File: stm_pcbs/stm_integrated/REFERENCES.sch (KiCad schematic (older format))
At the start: 20 parts, among them U13 AD8676, U14 AD8675, U15 ADR445

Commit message: working on Kicad of 3rd Dec
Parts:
- C65, C66, C69, C70, C71, C74: symbol CP2 -> device:CP1
- C67, C68, C72, C73, C75, C76: symbol C -> device:C
- R5, R6, R7, R8, R9: symbol R -> device:R
- U13: symbol AD8676 -> ad5791:AD8676
- U14: symbol AD8675 -> ad5791:AD8675
- U15: symbol adr445 -> adr445:adr445
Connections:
- wire segments 65 -> 81

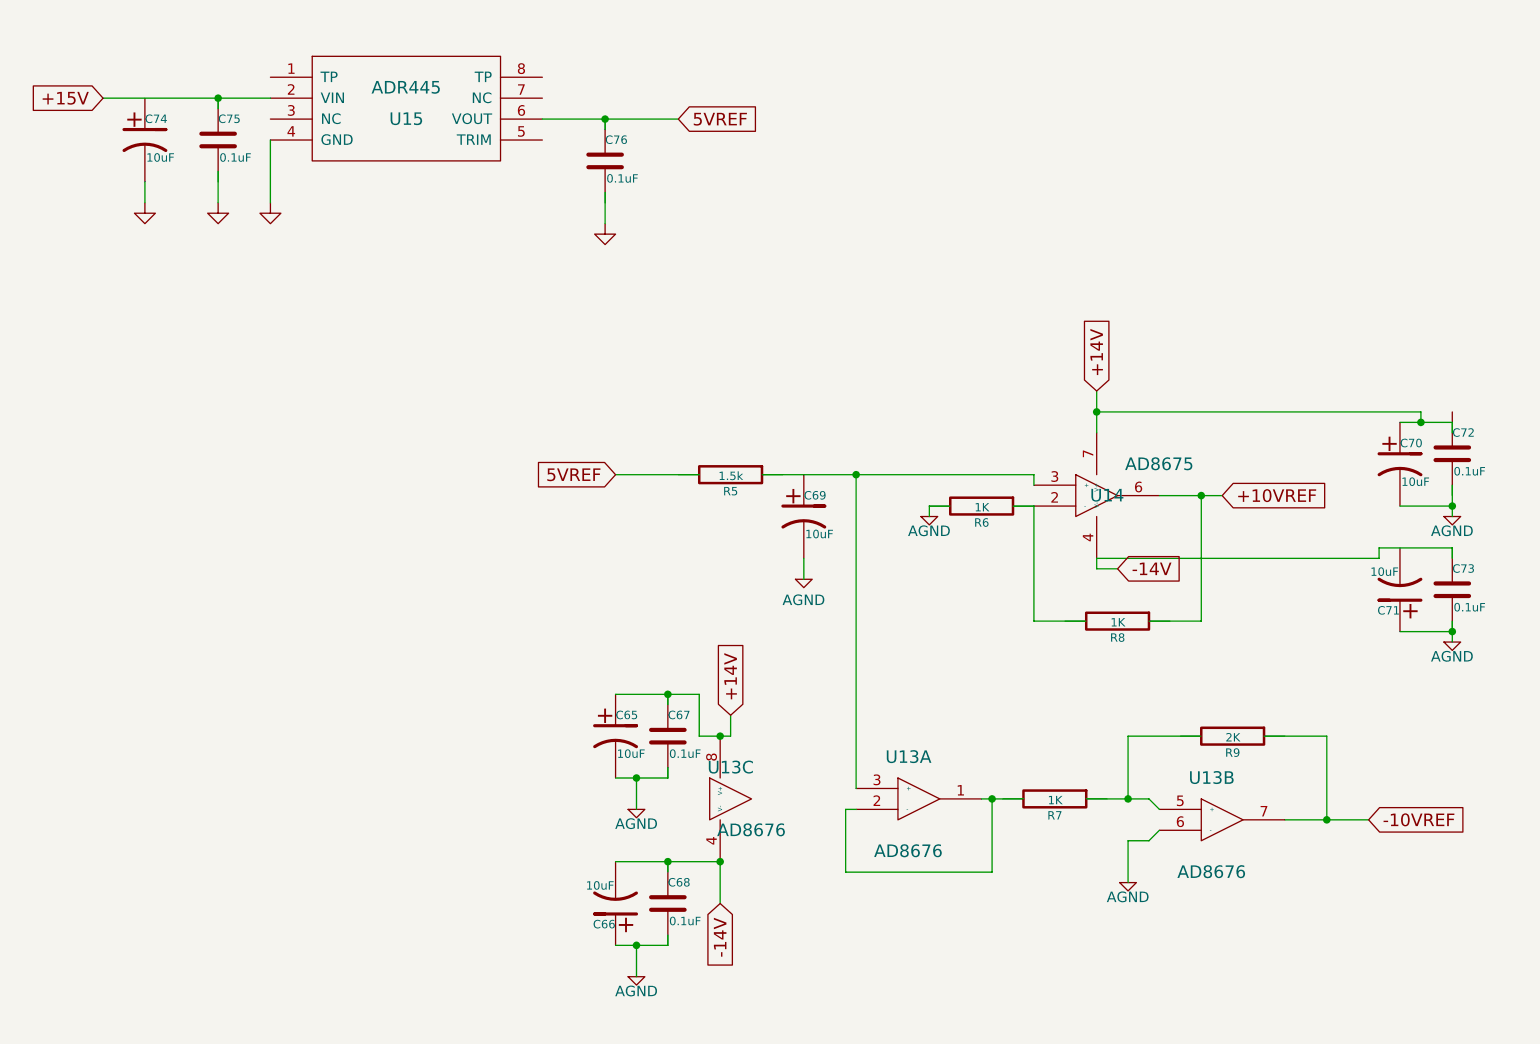
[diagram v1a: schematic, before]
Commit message: fixing more borkage
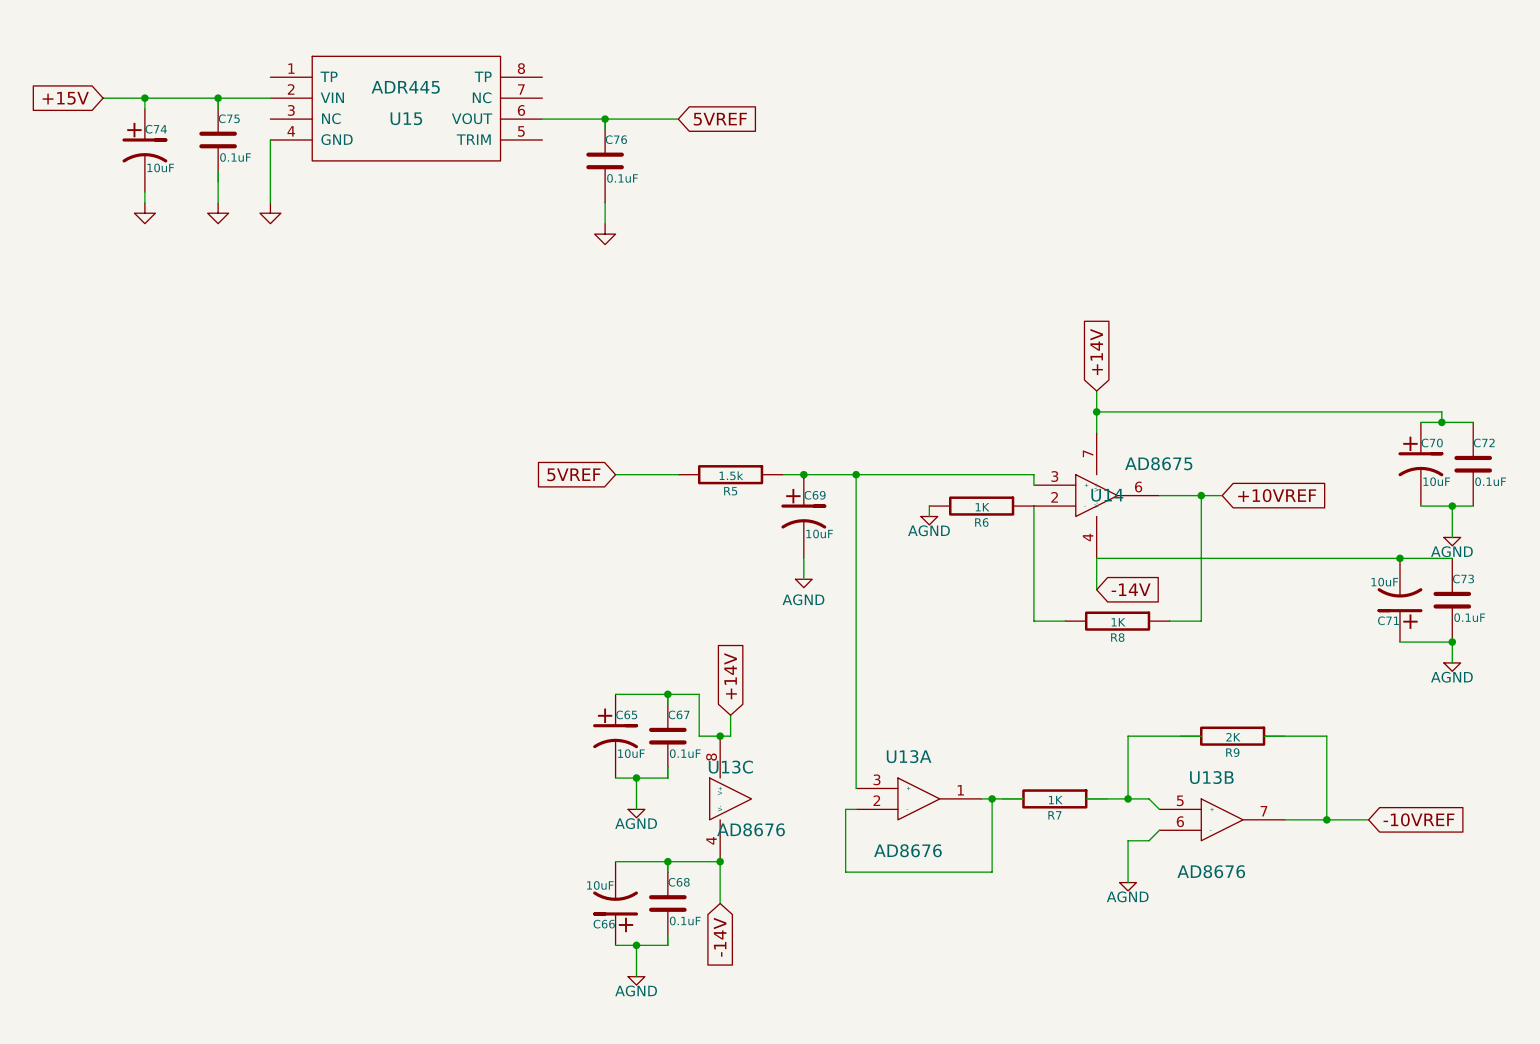
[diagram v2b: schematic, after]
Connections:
- wire segments 81 -> 77
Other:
- moved on the sheet: C70, C71, C72, C73, C74
